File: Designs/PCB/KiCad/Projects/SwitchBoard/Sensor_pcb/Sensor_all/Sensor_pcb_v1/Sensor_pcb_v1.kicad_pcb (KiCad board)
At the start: 2 copper layers, 32 parts, among them J1 Header 3x2, J2 Prog Hdr, J3 Solar_input, J4 SWD, J5 Battery_input, J6 Distance /, SW1 SW_Push, SW2 On/Off, U1 APK2112.K-3.3, U2 STM32, U3 LoRa, U4 BME_280, U5 Slide_switch, Y1 32.768K, Y2 8Mhz

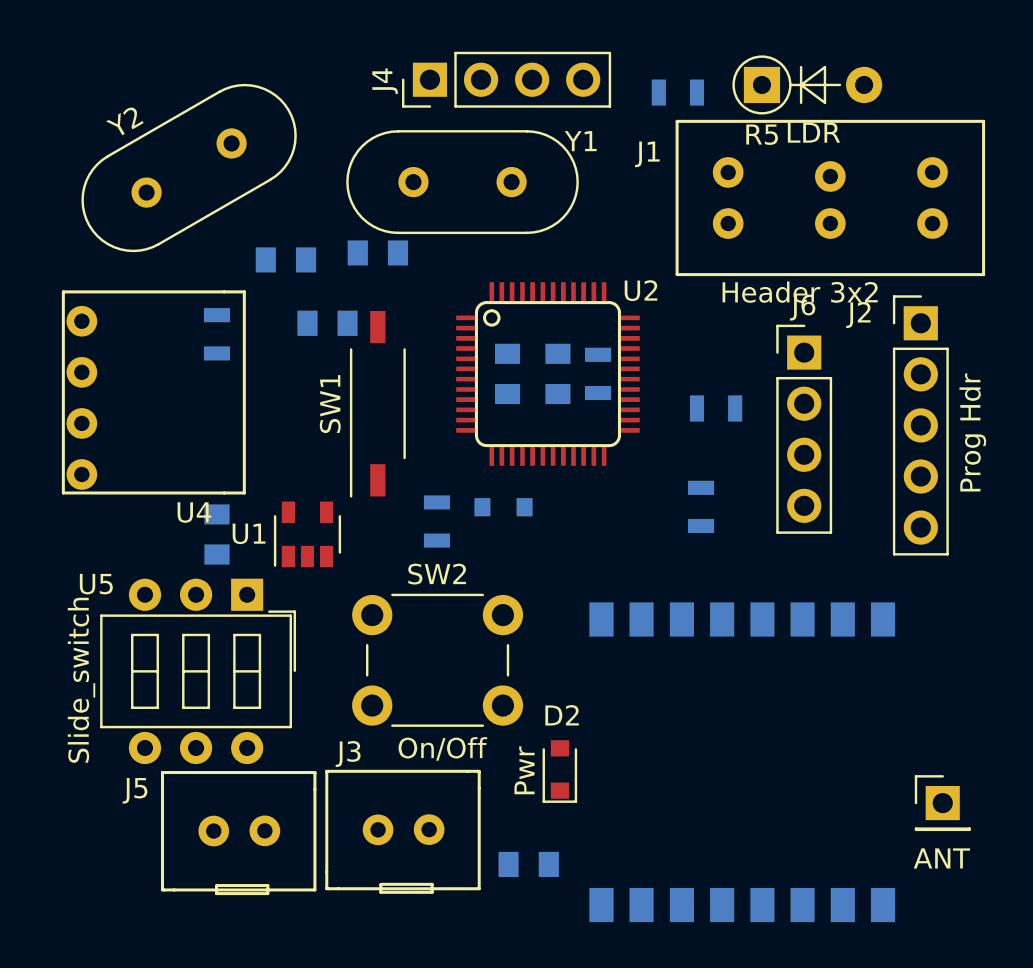
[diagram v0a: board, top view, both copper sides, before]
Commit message: update
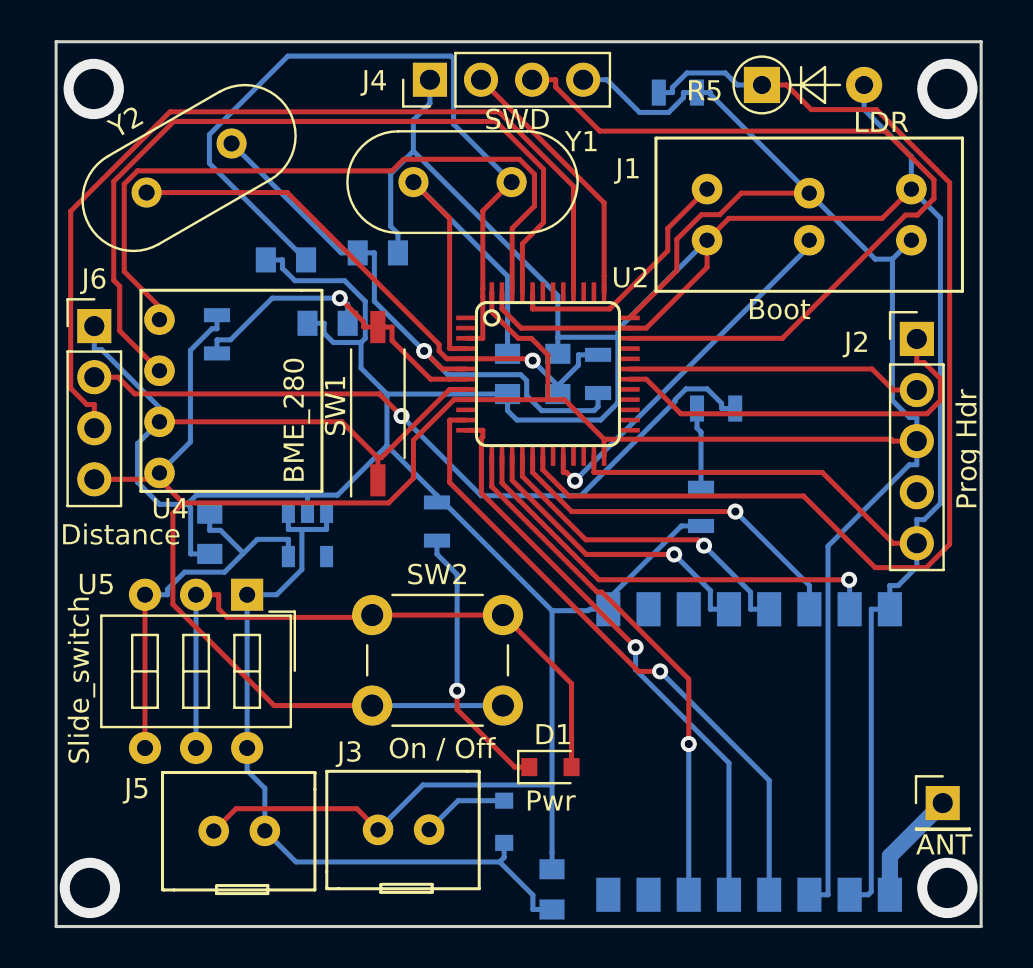
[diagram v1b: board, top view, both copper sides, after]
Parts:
- D1: value Pwr_L.E.D -> Pwr; moved to F.Cu
- D2: value Pwr -> DIODE; moved to B.Cu
- J1: value Header 3x2 -> Boot
- J6: value Distance / -> Distance
- SW2: value On/Off -> On / Off
- U1: moved to B.Cu
- moved J6 35.3 mm to (24.9, 32.7)
- moved D1 13.1 mm to (47.5, 54.6)
- moved U4 3.86 mm to (33.2, 34.9)
- moved D2 3.80 mm to (45.2, 57.4), turned to 270 degrees
- moved C6 1.70 mm to (47.6, 60.7), turned to 270 degrees
- moved J1 1.34 mm to (60.4, 25.9)
- moved J2 0.81 mm to (65.8, 33.3)
- moved U3 0.61 mm to (57.4, 57.5)
- moved C7 0.36 mm to (30.6, 43.0)
- turned U1 to 270 degrees
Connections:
- net /Touch_1 renamed Net-(U2-Pad10)
- net /Touch_2 renamed Net-(U2-Pad25)
- U2 pad 2: /Touch_3 -> Net-(U2-Pad2)
- U2 pad 26: /Touch_3 -> Net-(U2-Pad26)
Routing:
- net GNDREF: track 0.00 -> 254.2 mm
- net /VCC3V3: track 0.00 -> 155.5 mm
- net /LDR_IN: track 0.00 -> 58.7 mm
- net /Trig: track 0.00 -> 45.4 mm
- net /SWIO: track 0.00 -> 41.2 mm
- net /SCL: track 0.00 -> 40.5 mm
- net /PC14: track 0.00 -> 38.6 mm
- net /BAT_IN: track 0.00 -> 38.3 mm
- net /Echo: track 0.00 -> 37.1 mm, vias 0 -> 1
- net /SDA: track 0.00 -> 35.0 mm
- net /Slide: track 0.00 -> 32.8 mm
- net /Reset_LoRa: track 0.00 -> 31.6 mm, vias 0 -> 1
- net /DIO0: track 0.00 -> 29.1 mm, vias 0 -> 1
- net /OSCOUT: track 0.00 -> 28.8 mm, vias 0 -> 1
- net /OSCIN: track 0.00 -> 28.0 mm, vias 0 -> 1
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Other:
- board outline added: 46 x 44 mm
- rule trace_min: 0.2 -> 0.3
- rule via_min_size: 0.4 -> 4.5
